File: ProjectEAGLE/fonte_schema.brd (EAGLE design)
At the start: 47 x 37.8 mm, 10 parts, among them T1 2N3904

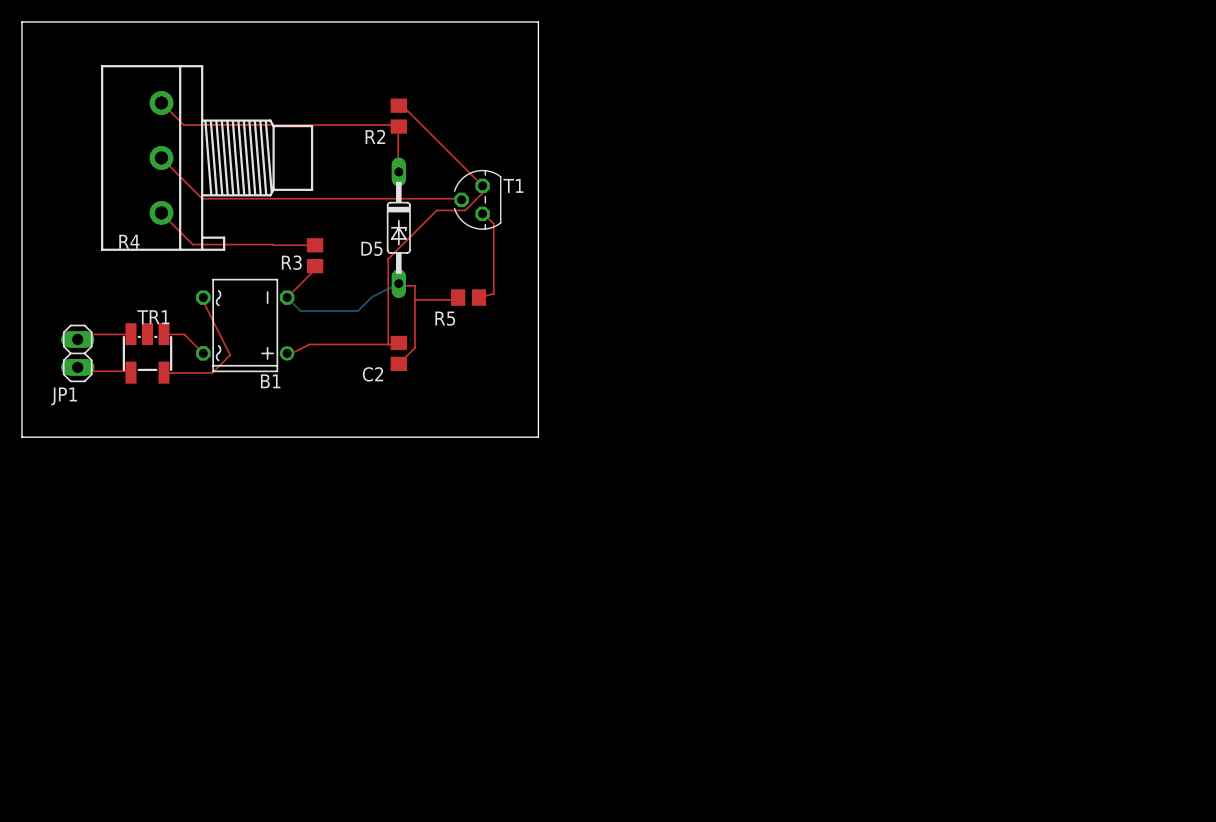
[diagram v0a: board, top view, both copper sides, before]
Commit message: Finalizando
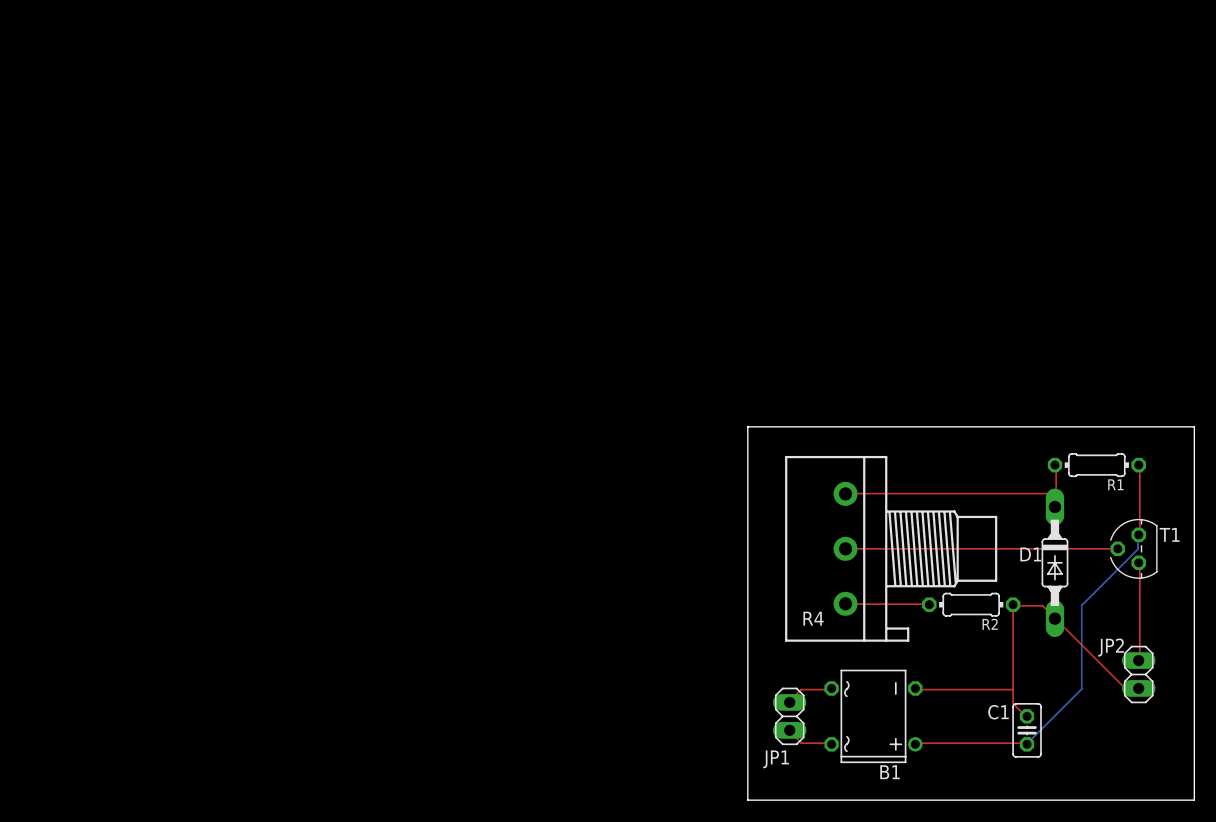
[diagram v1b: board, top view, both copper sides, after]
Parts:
- removed C2: 750u, rcl:C0805
- removed D5: 13v, diode:DO35Z10
- removed R3: 2.2k, rcl:R0805
- removed R5: 120, rcl:R0805
- removed TR1: 15V, inductor-neosid:SM-T4
- added C1: 750u, rcl:C025-025X050
- added D1: 13v, diode:SOD81
- added JP2: 3-12V, pinhead:1X02
- added R1: 330, rcl:0204/7
- JP1: value 127V -> 15V
- R2: value 330 -> 2.2k; device rcl:R0805 -> rcl:0204/7
- R4: value 4.7k -> 5k
- moved JP1 72.7 mm to (3.81, 7.62), turned to 270 degrees
- moved R4 71.7 mm to (8.89, 22.9)
- moved R2 68.5 mm to (20.3, 17.8), turned to 180 degrees
- moved T1 67.6 mm to (35.6, 22.9)
- moved B1 67.3 mm to (11.4, 7.62)
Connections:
- removed net N$10: JP1.2, TR1.2
- removed net N$9: JP1.1, TR1.1
- net N$1: now also JP2.2, T1.3; no longer B1.-, C2.2, D5.A, R3.1, R5.1
- net N$2: now also JP1.1; no longer TR1.5
- net N$3: now also C1.1, R1.1; no longer C2.1, R2.1
- net N$4: now also D1.C, R1.2; no longer D5.C, R2.2
- net N$5: now also JP1.2; no longer TR1.4
- net N$7: now also R2.2; no longer R3.2
- net N$8: now also B1.-, C1.2, D1.A, JP2.1, R2.1; no longer R5.2, T1.3
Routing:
- net N$8: track 9.13 -> 34.3 mm
- net N$1: track 28.7 -> 8.97 mm
- net N$2: track 12.5 -> 4.46 mm
- net N$7: track 15.2 -> 7.65 mm
- net N$9: track 5.07 -> 0.00 mm
- net N$10: track 5.04 -> 0.00 mm
- net N$6: track 28.9 -> 24.8 mm
- net N$4: track 26.7 -> 24.4 mm
- net N$3: track 40.6 -> 40.0 mm
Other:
- board size 47 x 37.8 mm -> 40.6 x 34 mm
